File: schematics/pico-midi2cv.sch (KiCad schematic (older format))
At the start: 33 parts, among them J1 Jack-DC (12-32V), U1 LM7805_TO220, U2 LM358, U3 MCP4822, U4 6N138

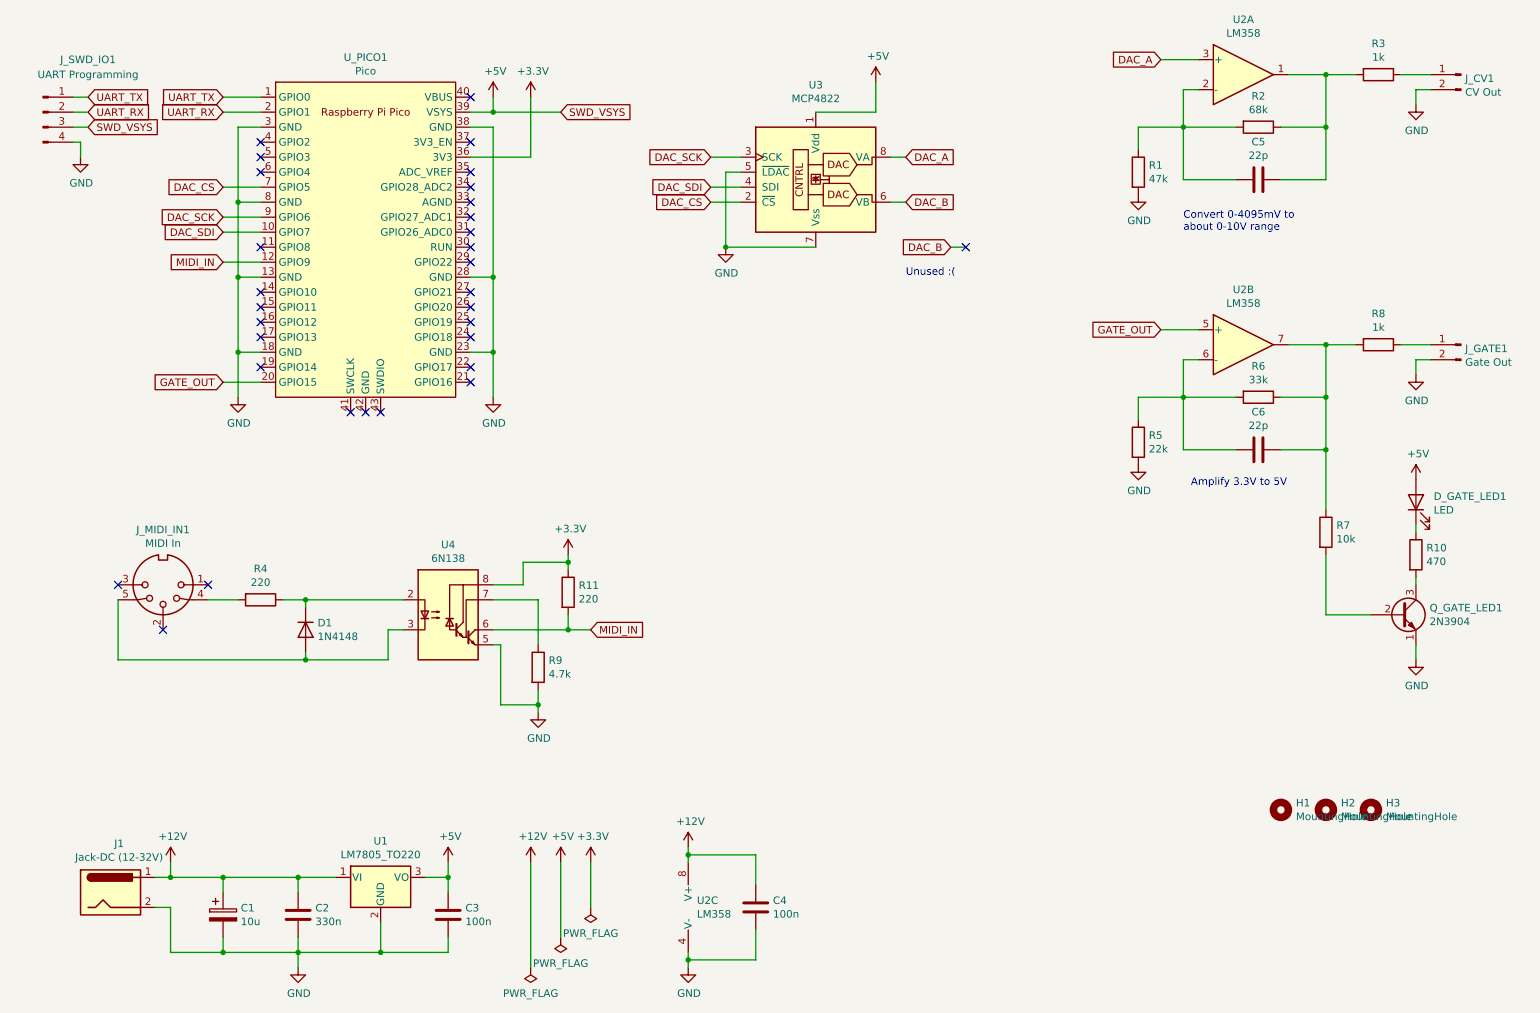
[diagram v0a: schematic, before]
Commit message: Updated schematics
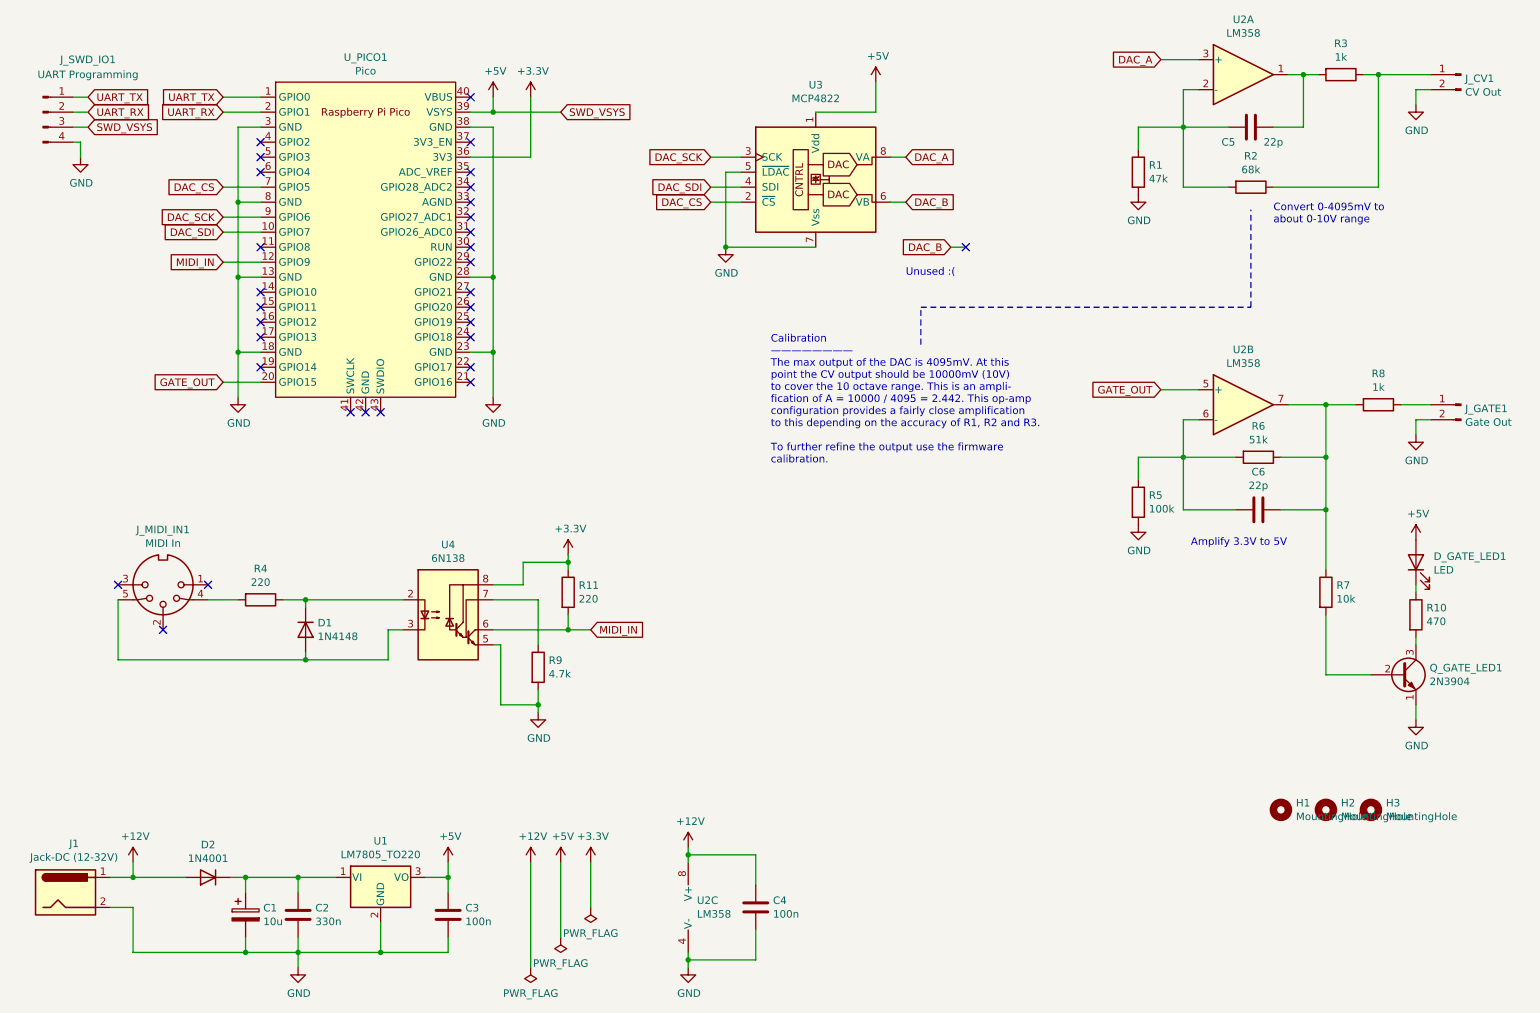
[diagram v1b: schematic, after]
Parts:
- added D2: 1N4001, Zimo_Manual_PCB:D_Axial, symbol Device:D
- R5: value 22k -> 100k
- R6: value 33k -> 51k
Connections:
- net +12V: now also D2.2 (A); no longer C1.1, C2.1, U1.1 (VI)
- net at C5.1, R3.2, U2.1: no longer R2.1
- net at J_CV1.1 (Pin_1), R3.1: now also R2.1
- new net: C1.1, C2.1, D2.1 (K), U1.1 (VI)
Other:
- note added: "Calibration\n————————\nThe max output of the DAC is 4095mV. At this\npoint the CV output should be 10000mV (10V)\nto cover the 10 octave range. This is an ampli-\nfication of A = 10000 / 4095 = 2.442. This op-amp\nconfiguration provides a fairly close amplification\nto this depending on the accuracy of R1, R2 and R3.\n\nTo further refine the output use the firmware\ncalibration."
- moved on the sheet: C1, C5, C6, D_GATE_LED1, J1, J_GATE1, Q_GATE_LED1, R10, R3, R5, R6, R7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
